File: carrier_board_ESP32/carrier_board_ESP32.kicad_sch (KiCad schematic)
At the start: 45 parts, among them IC1 SS49E, IC2 SS49E, IC3 SS49E, IC4 SS49E, IC5 SS49E, IC6 SS49E, IC7 DRV5023, IC8 DRV5023, J1 BME280, J2 LTR390, J3 ENS160 I2C, J4 ENS160 SPI, J5 ENS160 + AHT21, J6 Conn_01x02_Socket, J7 Conn_01x02_Socket, J8 UJC-HP-3-SMT-TR, U1 ESP32-S3-DEVKITC-1-N8R2, U2 TP4056, U3 LM2576HVS-5, U4 MT3608

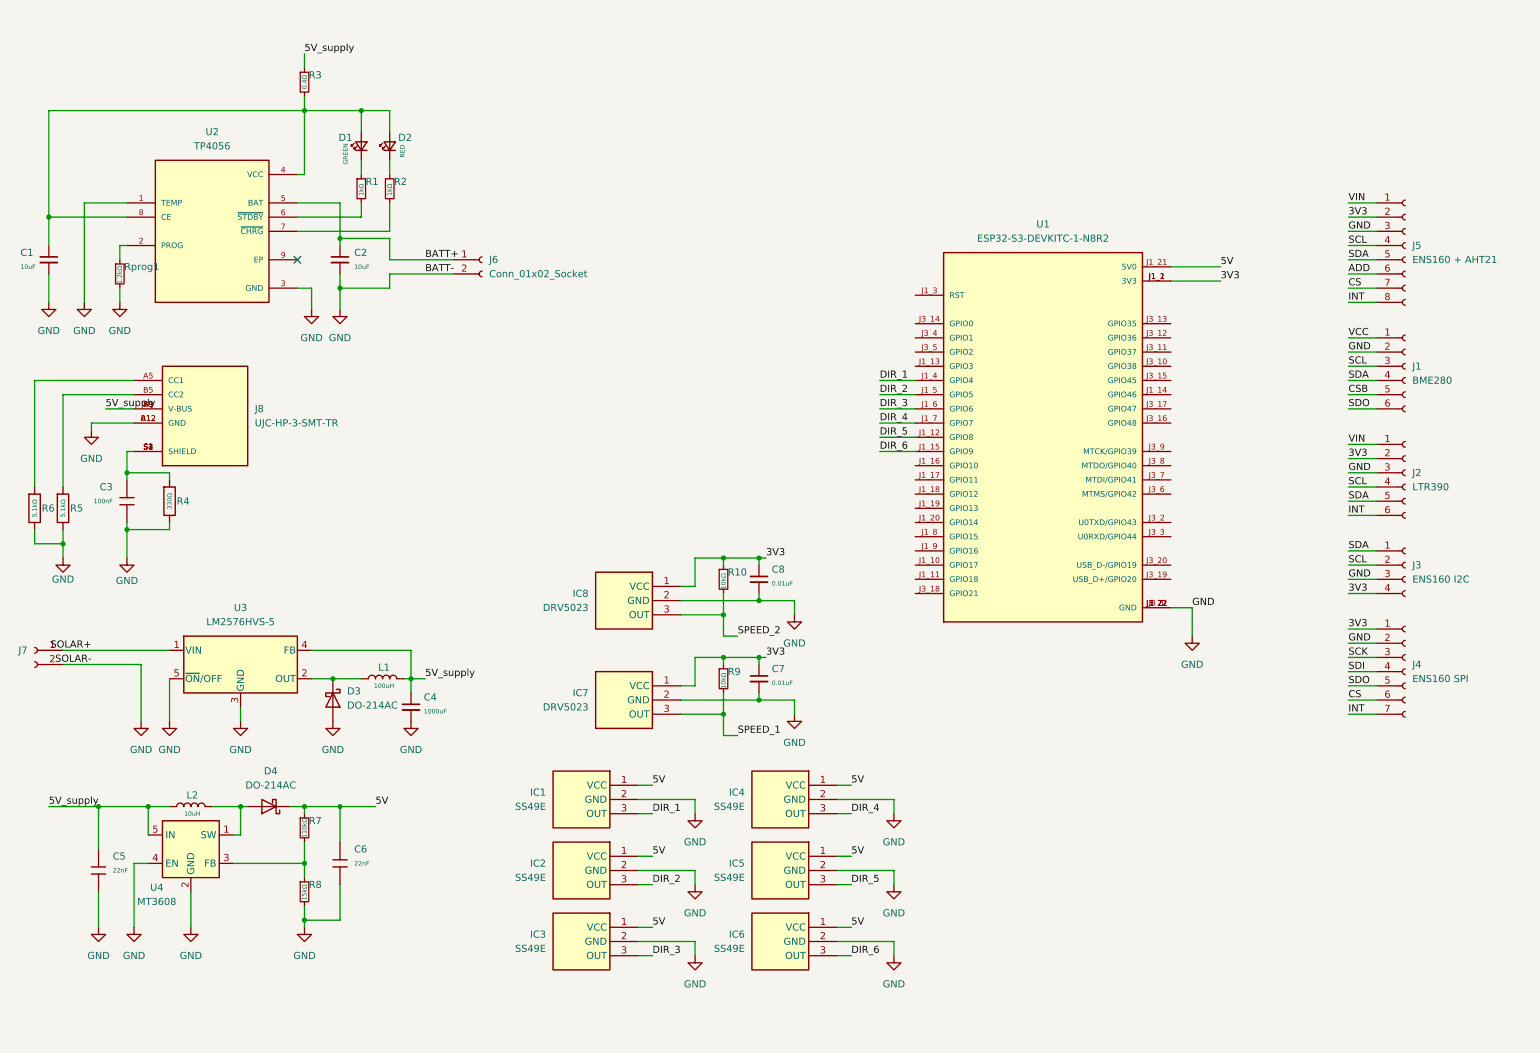
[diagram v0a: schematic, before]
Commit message: formated file, ready for check
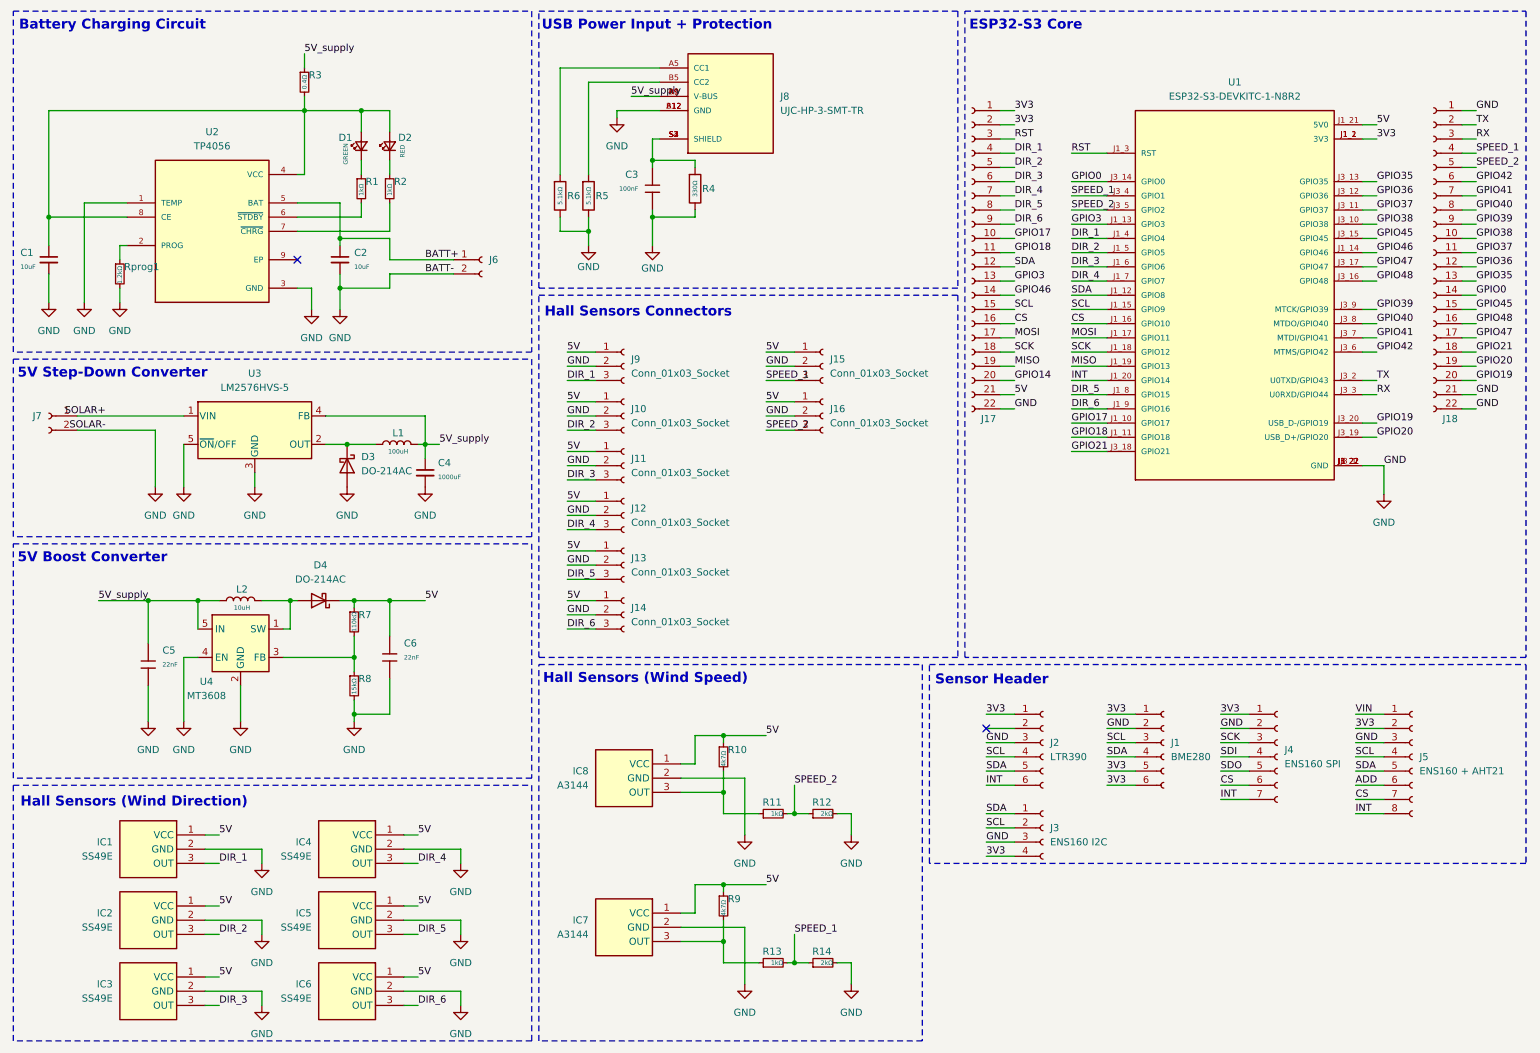
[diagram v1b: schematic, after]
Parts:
- removed C7, C8: 0.01uF, Capacitor_SMD:C_0805_2012Metric_Pad1.18x1.45mm_HandSolder, symbol Device:C_Small
- added J10, J11, J12, J13, J14, J15, J16, J9: Conn_01x03_Socket, Connector_PinHeader_2.54mm:PinHeader_1x03_P2.54mm_Vertical, symbol Connector:Conn_01x03_Socket
- added J17, J18: Conn_01x22_Socket, symbol Connector:Conn_01x22_Socket
- added R11, R13: 1kΩ, Resistor_SMD:R_0805_2012Metric_Pad1.20x1.40mm_HandSolder, symbol Device:R_Small
- added R12, R14: 2kΩ, Resistor_SMD:R_0805_2012Metric_Pad1.20x1.40mm_HandSolder, symbol Device:R_Small
- IC7, IC8: value DRV5023 -> A3144
- R10, R9: value 10kΩ -> 4k7Ω
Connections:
- net CSB is gone; now on net 3V3: J1.5 (Pin_5)
- net VCC is gone; now on net 3V3: J1.1 (Pin_1)
- net 3V3: now also J1.6 (Pin_6), J2.1 (Pin_1), J17.1 (Pin_1), J17.2 (Pin_2); no longer IC7.1 (VCC), IC8.1 (VCC), J2.2 (Pin_2), R10.1, R9.1
- net 5V: now also IC7.1 (VCC), IC8.1 (VCC), R10.1, R9.1, J10.1 (Pin_1), J11.1 (Pin_1), J12.1 (Pin_1), J13.1 (Pin_1), J14.1 (Pin_1), J15.1 (Pin_1), J16.1 (Pin_1), J17.21 (Pin_21), J9.1 (Pin_1)
- net CS: now also U1.J1_16 (GPIO10), J17.16 (Pin_16)
- net DIR_1: now also J17.4 (Pin_4), J9.3 (Pin_3)
- net DIR_2: now also J10.3 (Pin_3), J17.5 (Pin_5)
- net DIR_3: now also J11.3 (Pin_3), J17.6 (Pin_6)
- net DIR_4: now also J12.3 (Pin_3), J17.7 (Pin_7)
- net DIR_5: now also U1.J1_8 (GPIO15), J13.3 (Pin_3), J17.8 (Pin_8); no longer U1.J1_12 (GPIO8)
- net DIR_6: now also U1.J1_9 (GPIO16), J14.3 (Pin_3), J17.9 (Pin_9); no longer U1.J1_15 (GPIO9)
- net GND: now also J10.2 (Pin_2), J11.2 (Pin_2), J12.2 (Pin_2), J13.2 (Pin_2), J14.2 (Pin_2), J15.2 (Pin_2), J16.2 (Pin_2), J17.22 (Pin_22), J18.1 (Pin_1), J18.21 (Pin_21), J18.22 (Pin_22), J9.2 (Pin_2), R12.2, R14.2
- net INT: now also U1.J1_20 (GPIO14)
- net SCK: now also U1.J1_18 (GPIO12), J17.18 (Pin_18)
- net SCL: now also U1.J1_15 (GPIO9), J17.15 (Pin_15)
- net SDA: now also U1.J1_12 (GPIO8), J17.12 (Pin_12)
- net SDO: no longer J1.6 (Pin_6)
- net SPEED_1: now also U1.J3_4 (GPIO1), J15.3 (Pin_3), J18.4 (Pin_4), R13.2, R14.1; no longer IC7.3 (OUT), R9.2
- net SPEED_2: now also U1.J3_5 (GPIO2), J16.3 (Pin_3), J18.5 (Pin_5), R11.2, R12.1; no longer IC8.3 (OUT), R10.2
- net VIN: no longer J2.1 (Pin_1)
- net GPIO17: now reaches U1.J1_10 (GPIO17)
- net GPIO17: now also J17.10 (Pin_10)
- net GPIO18: now reaches U1.J1_11 (GPIO18)
- net GPIO18: now also J17.11 (Pin_11)
- net GPIO3: now reaches U1.J1_13 (GPIO3)
- net GPIO3: now also J17.13 (Pin_13)
- net GPIO46: now reaches U1.J1_14 (GPIO46)
- net GPIO46: now also J17.14 (Pin_14)
- net MOSI: now reaches U1.J1_17 (GPIO11)
- net MOSI: now also J17.17 (Pin_17)
- net MISO: now reaches U1.J1_19 (GPIO13)
- net MISO: now also J17.19 (Pin_19)
- net RST: now reaches U1.J1_3 (RST)
- net RST: now also J17.3 (Pin_3)
- net GPIO38: now reaches U1.J3_10 (GPIO38)
- net GPIO38: now also J18.10 (Pin_10)
- net GPIO37: now reaches U1.J3_11 (GPIO37)
- net GPIO37: now also J18.11 (Pin_11)
- net GPIO36: now reaches U1.J3_12 (GPIO36)
- net GPIO36: now also J18.12 (Pin_12)
- net GPIO35: now reaches U1.J3_13 (GPIO35)
- net GPIO35: now also J18.13 (Pin_13)
- net GPIO0: now reaches U1.J3_14 (GPIO0)
- net GPIO0: now also J18.14 (Pin_14)
- net GPIO45: now reaches U1.J3_15 (GPIO45)
- net GPIO45: now also J18.15 (Pin_15)
- net GPIO48: now reaches U1.J3_16 (GPIO48)
- net GPIO48: now also J18.16 (Pin_16)
- net GPIO47: now reaches U1.J3_17 (GPIO47)
- net GPIO47: now also J18.17 (Pin_17)
- net GPIO21: now reaches U1.J3_18 (GPIO21)
- net GPIO21: now also J18.18 (Pin_18)
- net GPIO20: now reaches U1.J3_19 (USB_D+/GPIO20)
- net GPIO20: now also J18.19 (Pin_19)
- net TX: now reaches U1.J3_2 (U0TXD/GPIO43)
- net TX: now also J18.2 (Pin_2)
- net GPIO19: now reaches U1.J3_20 (USB_D-/GPIO19)
- net GPIO19: now also J18.20 (Pin_20)
- net RX: now reaches U1.J3_3 (U0RXD/GPIO44)
- net RX: now also J18.3 (Pin_3)
- net GPIO42: now reaches U1.J3_6 (MTMS/GPIO42)
- net GPIO42: now also J18.6 (Pin_6)
- net GPIO41: now reaches U1.J3_7 (MTDI/GPIO41)
- net GPIO41: now also J18.7 (Pin_7)
- net GPIO40: now reaches U1.J3_8 (MTDO/GPIO40)
- net GPIO40: now also J18.8 (Pin_8)
- net GPIO39: now reaches U1.J3_9 (MTCK/GPIO39)
- net GPIO39: now also J18.9 (Pin_9)
- new net: IC7.3 (OUT), R13.1, R9.2
- new net: IC8.3 (OUT), R10.2, R11.1
- new net GPIO14: J17.20 (Pin_20)
- no-connect marks 1 -> 2
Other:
- note added: "5V Boost Converter"
- note added: "5V Step-Down Converter"
- note added: "Battery Charging Circuit"
- note added: "ESP32-S3 Core"
- note added: "Hall Sensors (Wind Direction)"
- note added: "Hall Sensors (Wind Speed)"
- note added: "Hall Sensors Connectors"
- note added: "Sensor Header"
- note added: "USB Power Input + Protection"
- company: (none) -> Adam Prystupa 275496
- title: (none) -> ESP32-S3 carrier board
- moved on the sheet: C3, C4, C5, C6, D3, D4, IC1, IC2, IC3, IC4, IC5, IC6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
